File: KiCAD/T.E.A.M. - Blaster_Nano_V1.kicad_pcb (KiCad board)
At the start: 2 copper layers, 55.2 x 35.2 mm, 50 parts, among them J1 USB_C_Receptacle_USB2.0_14P, J2 AKKU, J3 LED, J4 Taster, J5 Speaker, J6 Conn_02x03_Counter_Clockwise, Q1 FS8205A, U1 TP4056-42-ESOP8, U2 DW01A, U3 MT3608, U4 ATMEGA328P-AU, U5 CH340G, U6 DFR0299, Y1 Crystal_GND34, Y2 Crystal_GND34

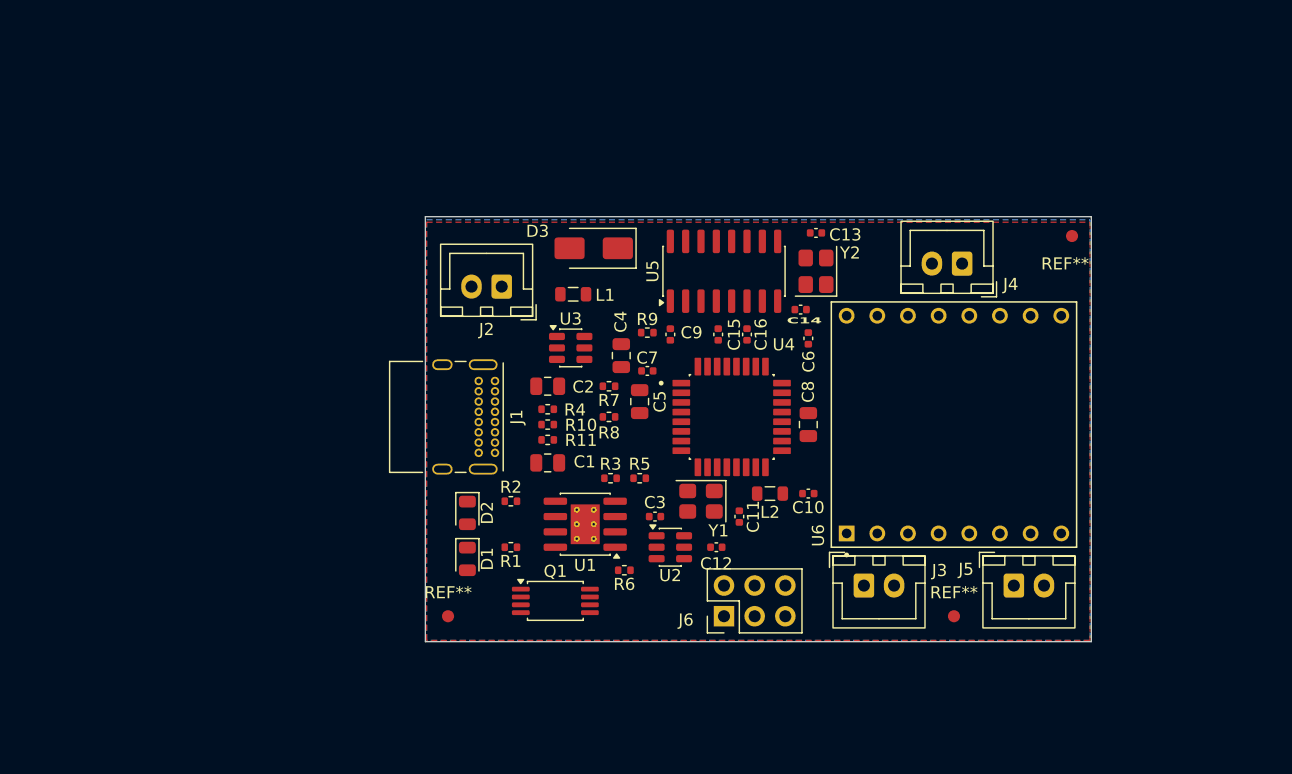
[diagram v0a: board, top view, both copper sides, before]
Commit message: PCB Routing Zwischenstand
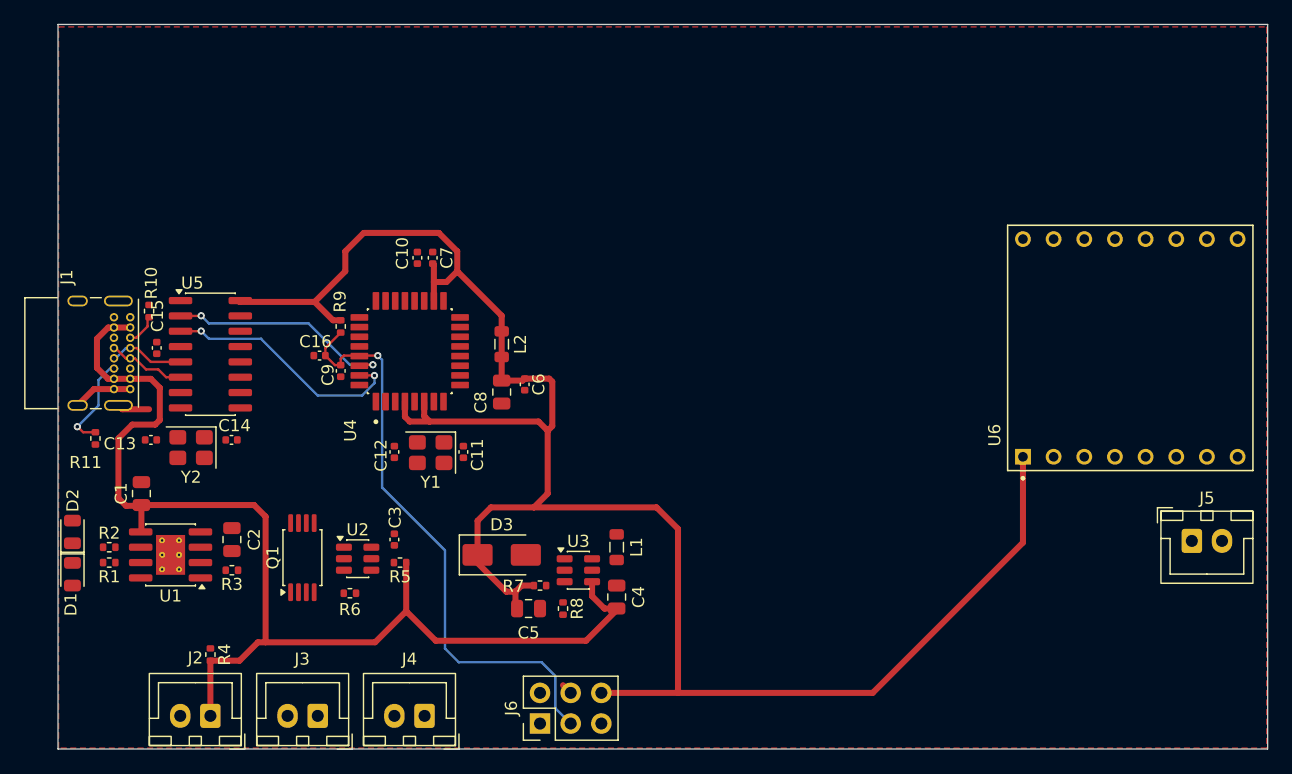
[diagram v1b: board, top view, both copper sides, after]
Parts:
- removed REF** (x3): Fiducial_1mm_Mask2mm, Fiducial:Fiducial_1mm_Mask2mm
- J2: value AKKU -> Akku
- moved J4 58.2 mm to (106.6, 118.7)
- moved C13 57.7 mm to (84.0, 95.9)
- moved Y2 53.8 mm to (87.3, 96.5), turned to 180 degrees
- moved C14 48.4 mm to (90.7, 95.9), turned to 180 degrees
- moved C15 46.5 mm to (84.5, 88.3)
- moved J3 46.5 mm to (97.8, 118.7), turned to 180 degrees
- moved U5 43.1 mm to (88.9, 88.8), turned to 0 degrees
- moved J2 43.0 mm to (88.9, 118.7)
- moved C10 37.8 mm to (106.0, 80.8), turned to -90 degrees
- moved R11 37.5 mm to (79.4, 95.8), turned to -90 degrees
- moved C16 35.4 mm to (97.9, 88.9), turned to 0 degrees
- moved R4 34.5 mm to (88.9, 113.7), turned to -90 degrees
- moved U1 34.4 mm to (85.6, 105.4)
- moved R10 34.3 mm to (83.8, 85.2), turned to 90 degrees
- moved C1 33.8 mm to (83.2, 100.3), turned to 90 degrees
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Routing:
- net VCC: track 0.00 -> 162.8 mm
- net VBATT: track 0.00 -> 98.5 mm
- net /RESET: track 0.00 -> 48.9 mm, vias 0 -> 1
- net /MCU_TX: track 0.00 -> 20.6 mm, vias 0 -> 2
- net /MCU_RX: track 0.00 -> 18.8 mm, vias 0 -> 2
- net GND: track 0.00 -> 8.49 mm
- net Net-(J1-CC2): track 0.00 -> 8.25 mm, vias 0 -> 1
- net /USB_DM: track 0.00 -> 6.52 mm
- net /USB_DP: track 0.00 -> 6.34 mm
- net Net-(J1-CC1): track 0.00 -> 2.64 mm
- removed copper zone on B.Cu, net GND
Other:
- board size 55.2 x 35.2 mm -> 100.2 x 60 mm
